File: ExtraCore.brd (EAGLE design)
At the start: 19.8 x 22.4 mm, 19 parts, among them Y1 RESONATORSMD

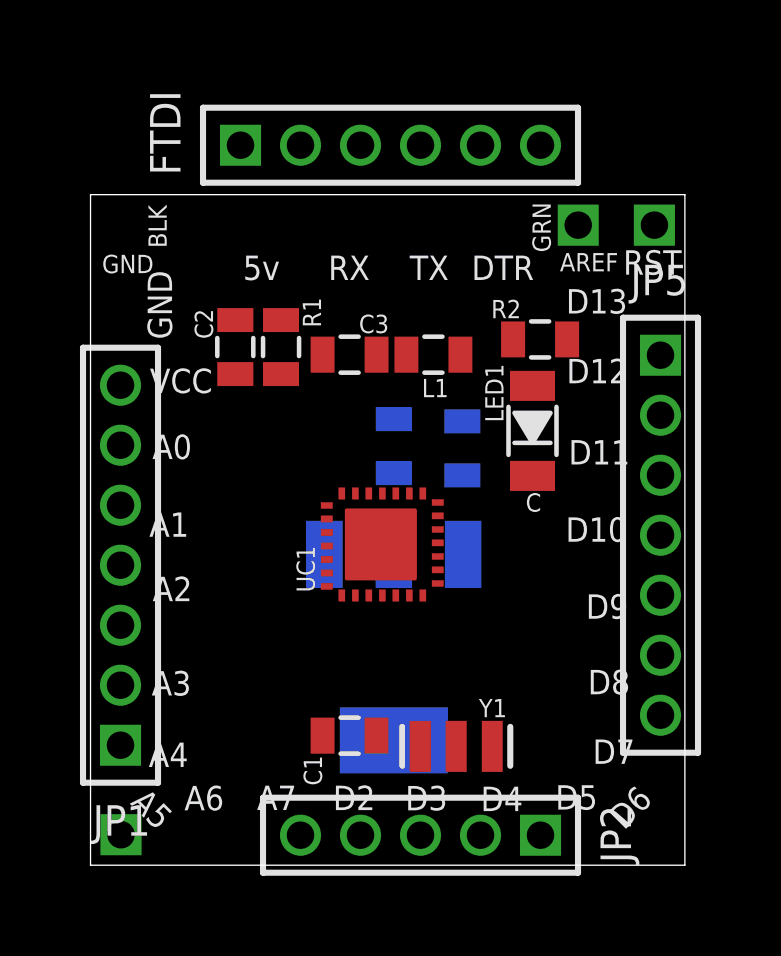
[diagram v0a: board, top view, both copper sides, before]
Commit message: moved stuff around. It's close to routable I think.
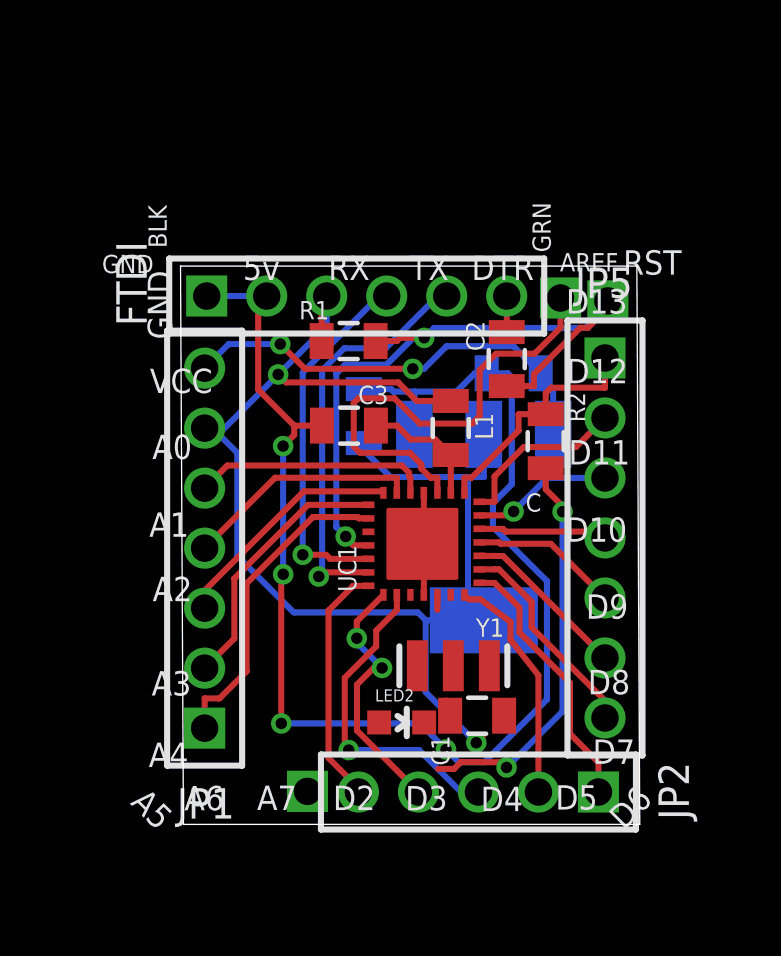
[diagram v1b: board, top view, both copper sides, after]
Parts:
- removed LED1: GREEN, ExtraCore:LED1206
- added LED2: (no value), SparkFun-LED:LED-0603
- moved C2 9.06 mm to (13.9, 16.9)
- moved A5 6.38 mm to (7.23, 2.46)
- moved FTDI 5.15 mm to (8.87, 19.0)
- moved RG1 5.00 mm to (13.1, 11.3)
- moved C1 4.30 mm to (12.9, 4.98)
- moved R2 3.40 mm to (15.2, 14.1), turned to 90 degrees
- moved C4 3.03 mm to (14.1, 16.4), turned to 0 degrees
- moved RESET 2.97 mm to (17.2, 18.8)
- moved JP1 2.86 mm to (3.80, 10.6)
- moved Y1 2.69 mm to (12.1, 6.65)
- moved L1 2.51 mm to (12.0, 14.6), turned to 90 degrees
- moved AREF 2.50 mm to (15.7, 18.9)
- moved JP2 2.41 mm to (12.9, 2.44)
- moved C3 2.37 mm to (8.61, 14.7)
- moved R1 2.26 mm to (8.60, 17.5), turned to 180 degrees
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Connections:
- net GND: now also LED2.C; no longer LED1.K
- net N$6: now also LED2.A; no longer LED1.A
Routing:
- net GND: track 0.00 -> 47.2 mm, vias 0 -> 4
- net VCC: track 0.00 -> 43.7 mm, vias 0 -> 2
- net RESET: track 0.00 -> 23.2 mm, vias 0 -> 2
- net AREF: track 0.00 -> 15.8 mm
- net RAW: track 0.00 -> 14.8 mm, vias 0 -> 2
- net TX: track 0.00 -> 13.8 mm, vias 0 -> 1
- net N$6: track 0.00 -> 13.4 mm, vias 0 -> 2
- net RX: track 0.00 -> 12.2 mm, vias 0 -> 1
- net D4: track 0.00 -> 10.8 mm, vias 0 -> 1
- net A4: track 0.00 -> 10.7 mm
- net D6: track 0.00 -> 8.91 mm
- net A3: track 0.00 -> 8.88 mm
- net D3: track 0.00 -> 8.65 mm, vias 0 -> 2
- net SCK: track 0.00 -> 8.16 mm
- net D2: track 0.00 -> 8.13 mm
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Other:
- board size 19.8 x 22.4 mm -> 15.3 x 18.6 mm
